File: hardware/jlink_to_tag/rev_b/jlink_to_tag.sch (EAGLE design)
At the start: 12 parts, among them J2 JLINK_6PIN_TAG-CON, U1 LT1763CS8-3.3

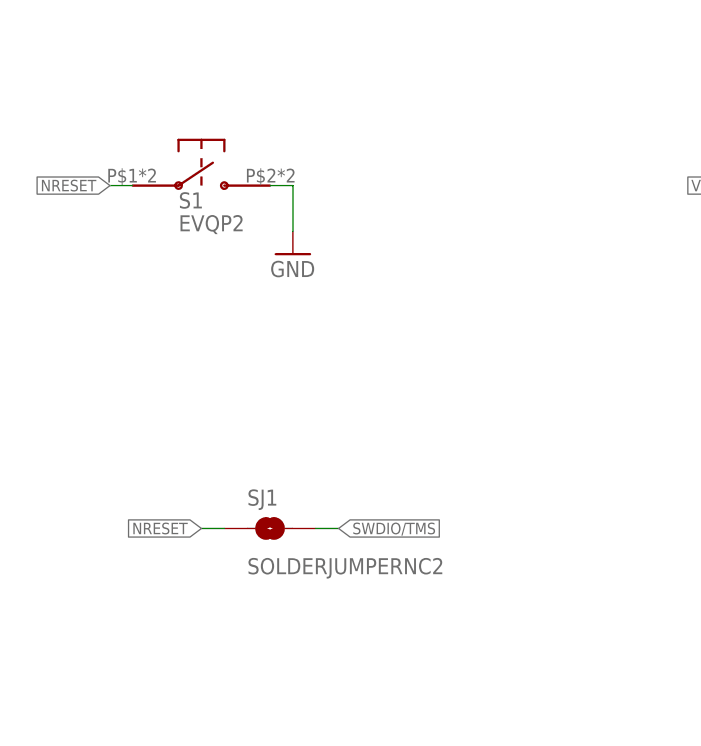
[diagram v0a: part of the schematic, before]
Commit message: revert rev b to the version that was fabbed
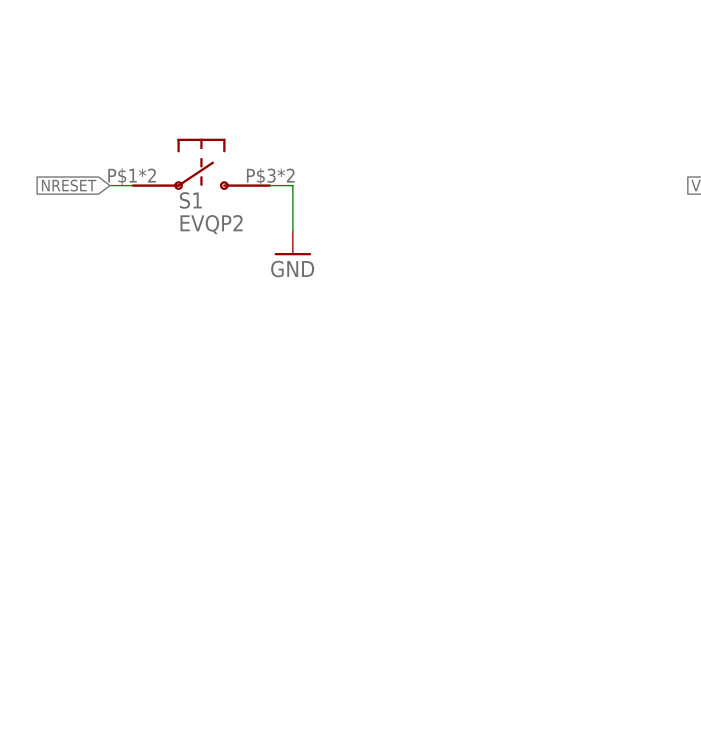
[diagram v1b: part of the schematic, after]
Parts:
- removed SJ1: SOLDERJUMPERNC2, SparkFun-Passives:SOLDERJUMPERNC2
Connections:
- net NRESET: no longer SJ1.1
- net SWDIO/TMS: no longer SJ1.2
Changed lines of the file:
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@@
 <part name="S2" library="switches" deviceset="TE_SSA12/SPDT" device=""/>
 <part name="GND3" library="SparkFun-Aesthetics" deviceset="GND" device=""/>
-<part name="SJ1" library="SparkFun-Passives" deviceset="SOLDERJUMPER" device="NC2"/>
 </parts>
 <sheets>
@@
 <instance part="S2" gate="G$1" x="101.6" y="83.82"/>
 <instance part="GND3" gate="1" x="45.72" y="76.2"/>
-<instance part="SJ1" gate="1" x="43.18" y="45.72"/>
 </instances>
 <busses>
@@
 <label x="25.4" y="83.82" size="1.27" layer="95" rot="R180" xref="yes"/>
 </segment>
-<segment>
-<pinref part="SJ1" gate="1" pin="1"/>
-<wire x1="38.1" y1="45.72" x2="35.56" y2="45.72" width="0.1524" layer="91"/>
-<label x="35.56" y="45.72" size="1.27" layer="95" rot="R180" xref="yes"/>
-</segment>
 </net>
 <net name="SWCLK/TCK" class="0">
@@
 <label x="45.72" y="134.62" size="1.27" layer="95" xref="yes"/>
 </segment>
-<segment>
-<pinref part="SJ1" gate="1" pin="2"/>
-<wire x1="48.26" y1="45.72" x2="50.8" y2="45.72" width="0.1524" layer="91"/>
-<label x="50.8" y="45.72" size="1.27" layer="95" xref="yes"/>
-</segment>
-</net>
+</net>

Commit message: bug fixes to rev b
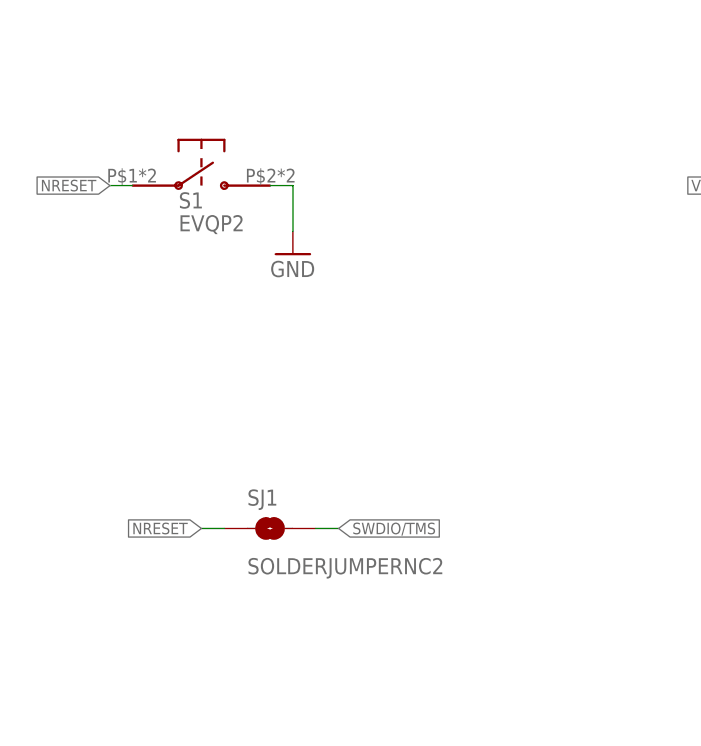
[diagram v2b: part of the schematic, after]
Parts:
- added SJ1: SOLDERJUMPERNC2, SparkFun-Passives:SOLDERJUMPERNC2
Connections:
- net NRESET: now also SJ1.1
- net SWDIO/TMS: now also SJ1.2
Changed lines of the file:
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@@
 <part name="S2" library="switches" deviceset="TE_SSA12/SPDT" device=""/>
 <part name="GND3" library="SparkFun-Aesthetics" deviceset="GND" device=""/>
+<part name="SJ1" library="SparkFun-Passives" deviceset="SOLDERJUMPER" device="NC2"/>
 </parts>
 <sheets>
@@
 <instance part="S2" gate="G$1" x="101.6" y="83.82"/>
 <instance part="GND3" gate="1" x="45.72" y="76.2"/>
+<instance part="SJ1" gate="1" x="43.18" y="45.72"/>
 </instances>
 <busses>
@@
 <label x="25.4" y="83.82" size="1.27" layer="95" rot="R180" xref="yes"/>
 </segment>
+<segment>
+<pinref part="SJ1" gate="1" pin="1"/>
+<wire x1="38.1" y1="45.72" x2="35.56" y2="45.72" width="0.1524" layer="91"/>
+<label x="35.56" y="45.72" size="1.27" layer="95" rot="R180" xref="yes"/>
+</segment>
 </net>
 <net name="SWCLK/TCK" class="0">
@@
 <label x="45.72" y="134.62" size="1.27" layer="95" xref="yes"/>
 </segment>
-</net>
+<segment>
+<pinref part="SJ1" gate="1" pin="2"/>
+<wire x1="48.26" y1="45.72" x2="50.8" y2="45.72" width="0.1524" layer="91"/>
+<label x="50.8" y="45.72" size="1.27" layer="95" xref="yes"/>
+</segment>
+</net>
